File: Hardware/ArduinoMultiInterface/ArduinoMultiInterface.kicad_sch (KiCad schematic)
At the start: 27 parts, among them J1 PORT1, J2 I2C, J3 SPI, J4 SER, SW1 SW_RESET, U1 ATmega328-P, U2 74HC165, U3 74HC595, U4 74HC574, U5 74HC574, U6 74HC574, U7 74HC04, U9 74LS20, Y1 20MHz

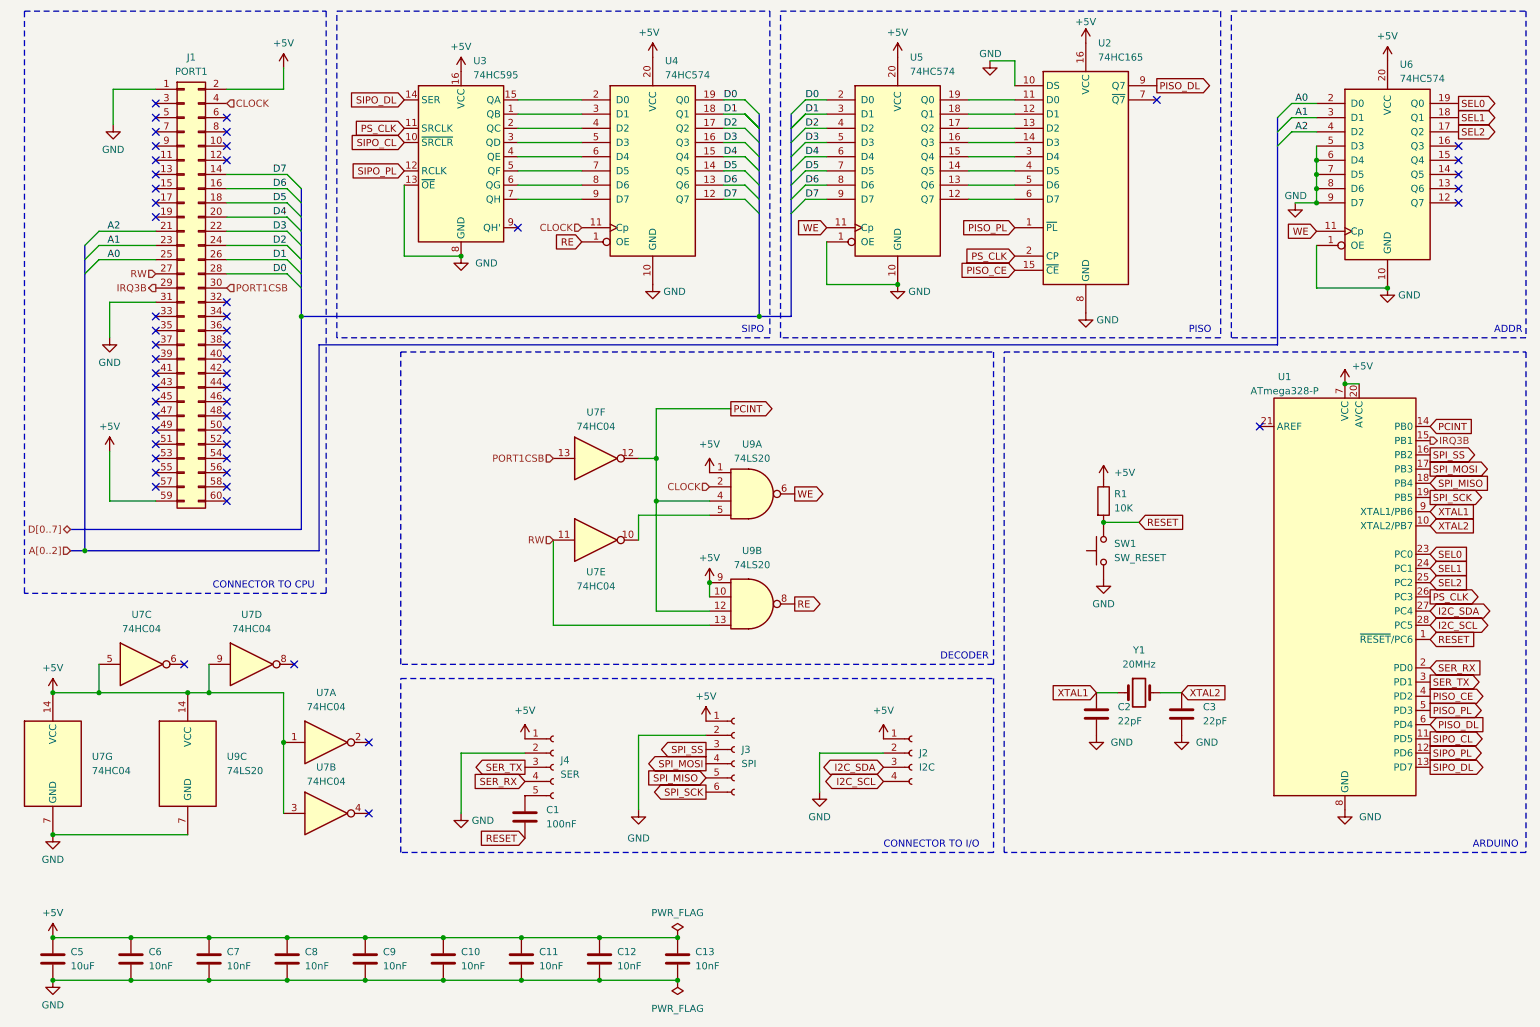
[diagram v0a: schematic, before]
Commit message: Add ArduinoMultiInterface
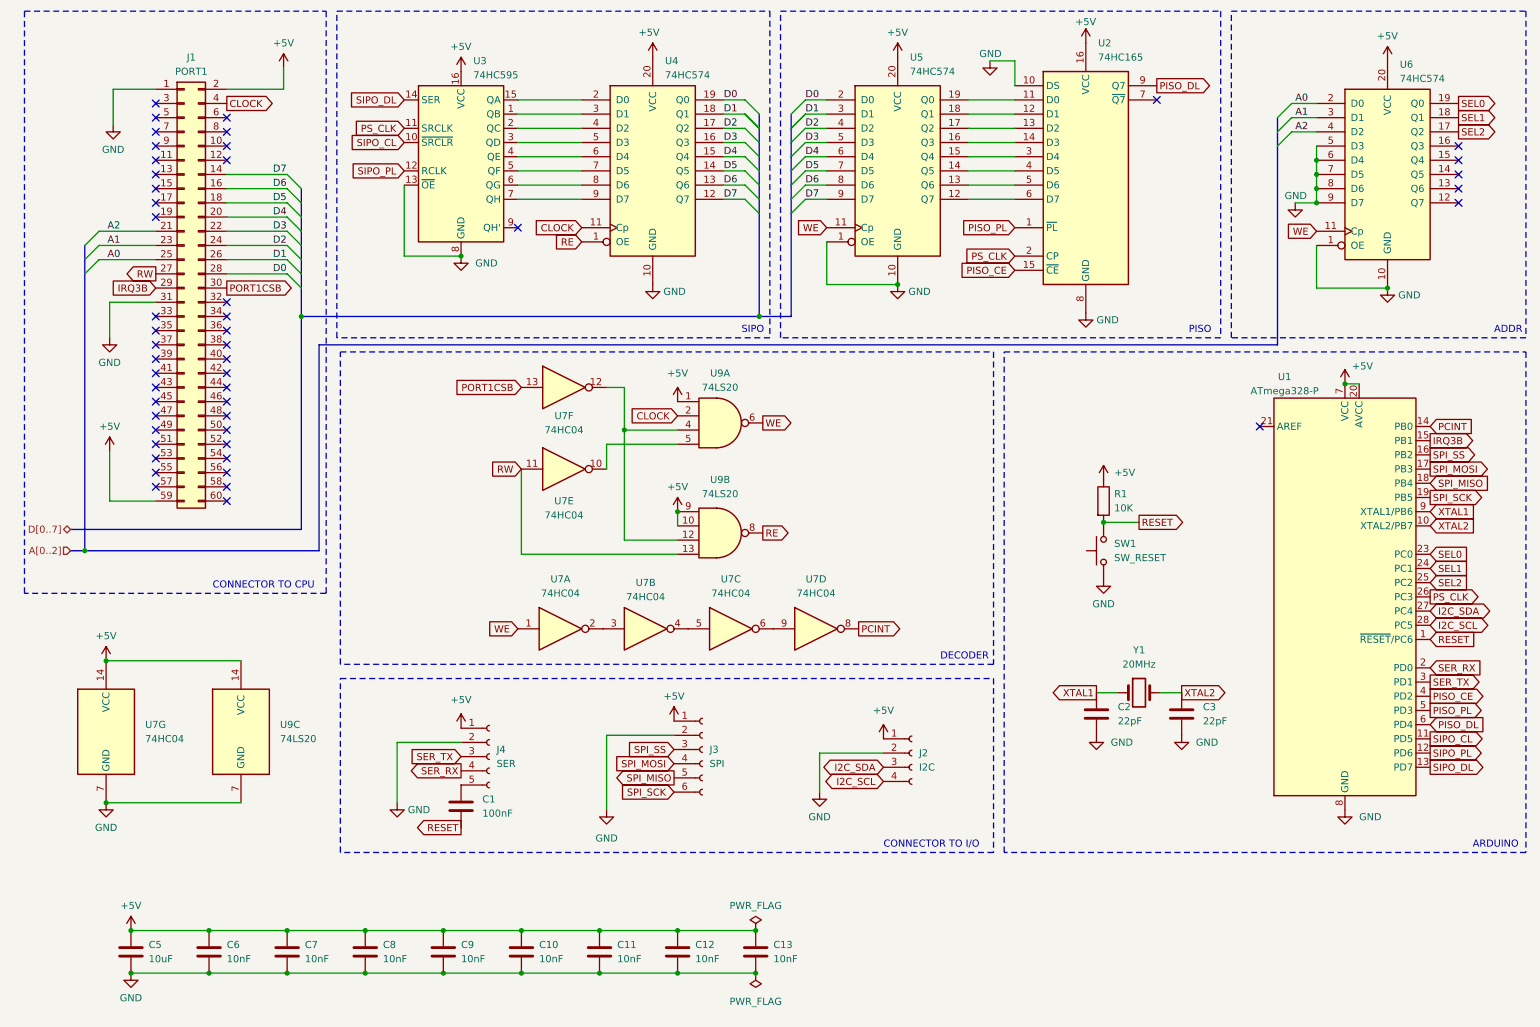
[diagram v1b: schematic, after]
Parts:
- Y1: footprint Crystal:Crystal_HC18-U_Vertical -> Crystal:Crystal_HC49-4H_Vertical
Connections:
- net +5V: no longer U7.1, U7.3, U7.5, U7.9
- net PCINT: now also U7.8; no longer U7.12, U9.12, U9.4
- net WE: now also U7.1
- net at U7.6: now also U7.9
- net at U7.2: now also U7.3
- net at U7.4: now also U7.5
- new net: U7.12, U9.12, U9.4
- no-connect marks 53 -> 49
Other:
- moved on the sheet: C1, C10, C11, C12, C13, C5, C6, C7, C8, C9, J3, J4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
